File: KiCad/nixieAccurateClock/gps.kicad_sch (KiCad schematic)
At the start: 5 parts, among them J5 Conn_Coaxial, J6 Conn_01x02_Pin, U4 PX1125T

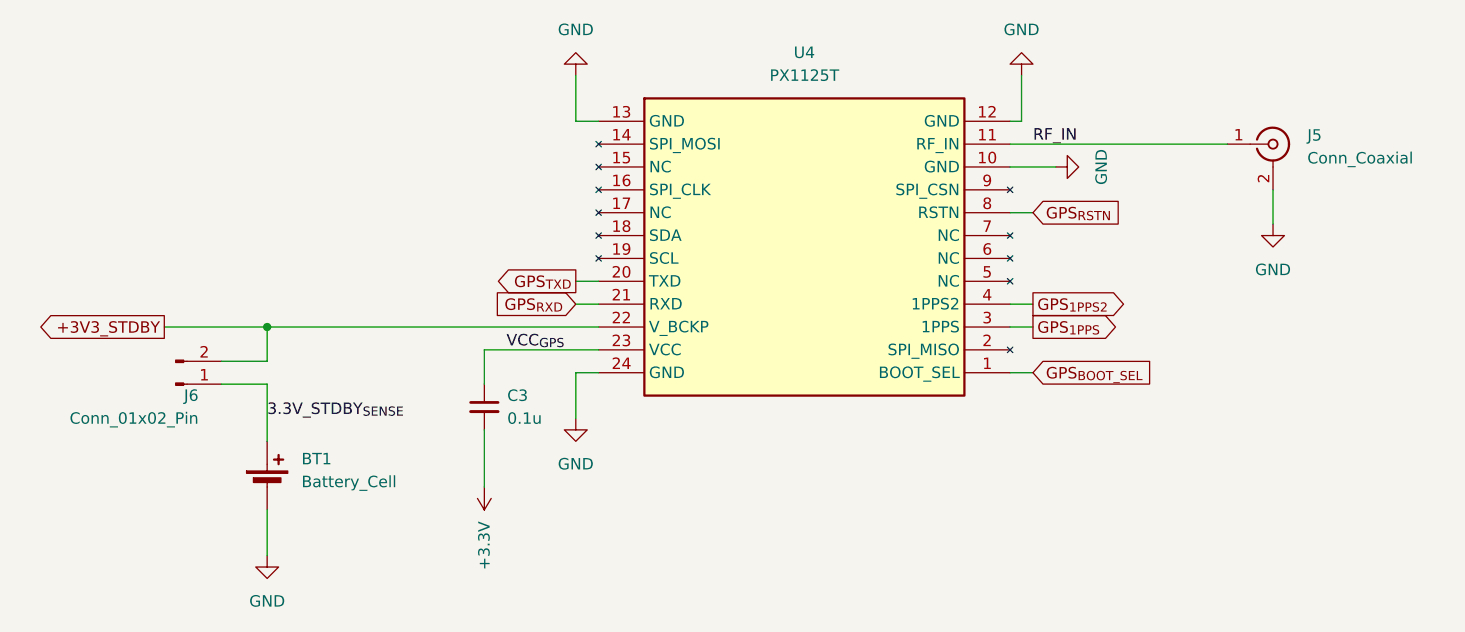
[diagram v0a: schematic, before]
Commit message: switch to 27k R_anode
Add voltage rail jumpers for different 5V and 3.3V standby applications
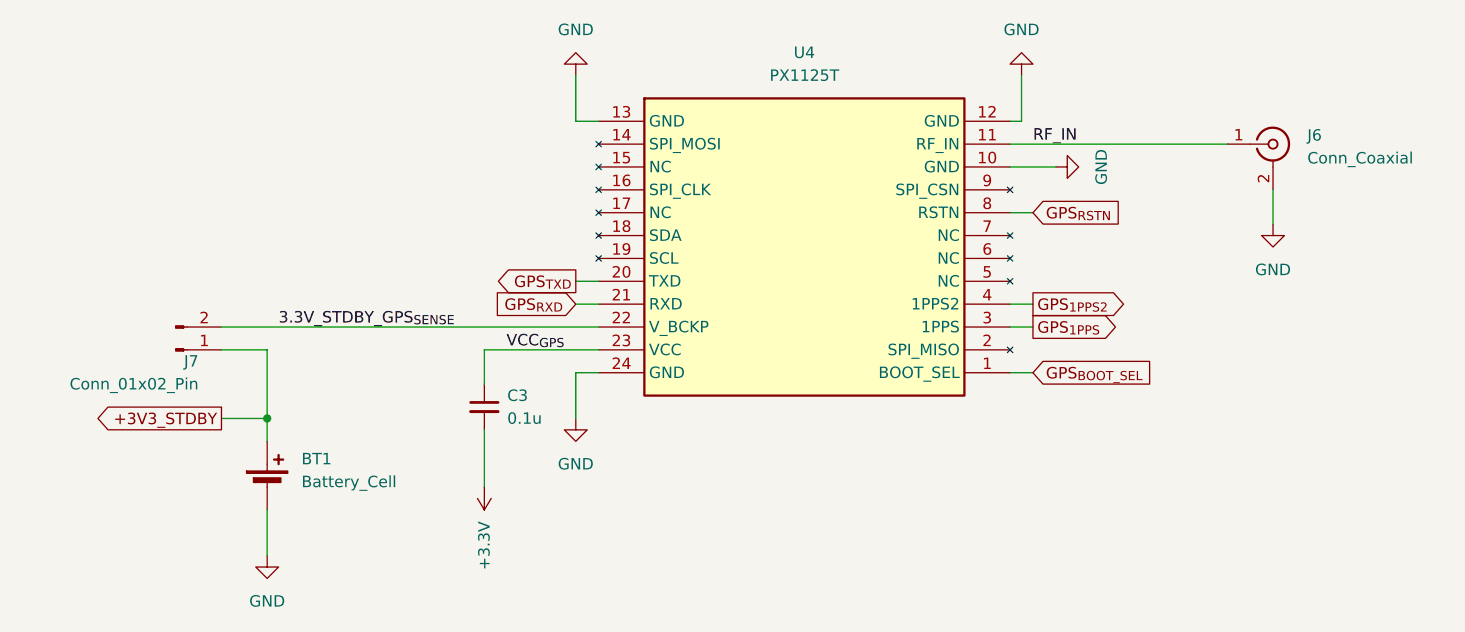
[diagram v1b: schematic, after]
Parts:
- renumbered J5 to J6, J6 to J7
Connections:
- net 3.3V_STDBY_{SENSE} is gone; now on net +3V3_STDBY: BT1.1 (+), J7.1 (Pin_1)
- net +3V3_STDBY: no longer J7.2 (Pin_2), U4.22 (V_BCKP)
- new net 3.3V_STDBY_GPS_{SENSE}: J7.2 (Pin_2), U4.22 (V_BCKP)
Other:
- moved on the sheet: J7
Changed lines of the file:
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@@
     (company "Paul Willis")
   )
-  (junction (at 72.39 110.49) (diameter 0) (color 0 0 0 0)
+  (junction (at 72.39 120.65) (diameter 0) (color 0 0 0 0)
   )
   (wire (pts (xy 184.15 95.25) (xy 184.15 99.06))
@@
     (stroke (width 0) (type default))
   )
-  (wire (pts (xy 72.39 110.49) (xy 109.22 110.49))
-    (stroke (width 0) (type default))
-  )
-  (wire (pts (xy 60.96 110.49) (xy 72.39 110.49))
-    (stroke (width 0) (type default))
-  )
   (wire (pts (xy 154.94 87.63) (xy 156.21 87.63))
     (stroke (width 0) (type default))
   )
-  (wire (pts (xy 72.39 114.3) (xy 72.39 110.49))
-    (stroke (width 0) (type default))
-  )
   (wire (pts (xy 72.39 130.81) (xy 72.39 135.89))
     (stroke (width 0) (type default))
@@
     (stroke (width 0) (type default))
   )
+  (wire (pts (xy 67.31 120.65) (xy 72.39 120.65))
+    (stroke (width 0) (type default))
+  )
+  (wire (pts (xy 67.31 110.49) (xy 109.22 110.49))
+    (stroke (width 0) (type default))
+  )
   (wire (pts (xy 154.94 110.49) (xy 157.48 110.49))
     (stroke (width 0) (type default))
@@
     (stroke (width 0) (type default))
   )
-  (wire (pts (xy 72.39 116.84) (xy 67.31 116.84))
-    (stroke (width 0) (type default))
-  )
-  (wire (pts (xy 67.31 114.3) (xy 72.39 114.3))
+  (wire (pts (xy 72.39 113.03) (xy 67.31 113.03))
+    (stroke (width 0) (type default))
+  )
+  (wire (pts (xy 72.39 120.65) (xy 72.39 123.19))
     (stroke (width 0) (type default))
   )
@@
     (stroke (width 0) (type default))
   )
-  (wire (pts (xy 72.39 116.84) (xy 72.39 123.19))
+  (wire (pts (xy 72.39 113.03) (xy 72.39 120.65))
     (stroke (width 0) (type default))
   )
@@
     (effects (font (size 1.27 1.27)) (justify right bottom))
   )
-  (label "3.3V_STDBY_{SENSE}" (at 72.39 120.65 0) (fields_autoplaced)
+  (label "3.3V_STDBY_GPS_{SENSE}" (at 73.66 110.49 0) (fields_autoplaced)
     (effects (font (size 1.27 1.27)) (justify left bottom))
   )
@@
     )
   )
-  (global_label "+3V3_STDBY" (shape output) (at 60.96 110.49 180) (fields_autoplaced)
+  (global_label "+3V3_STDBY" (shape output) (at 67.31 120.65 180) (fields_autoplaced)
     (effects (font (size 1.27 1.27)) (justify right))
-    (property "Intersheetrefs" "${INTERSHEET_REFS}" (at 46.1215 110.49 0)
+    (property "Intersheetrefs" "${INTERSHEET_REFS}" (at 52.4715 120.65 0)
       (effects (font (size 1.27 1.27)) (justify right) hide)
     )
@@
     )
   )
-  (symbol (lib_id "Connector:Conn_01x02_Pin") (at 62.23 116.84 0) (mirror x) (unit 1)
-    (in_bom yes) (on_board yes) (dnp no)
-    (property "Reference" "J6" (at 64.77 118.11 0)
+  (symbol (lib_id "Connector:Conn_01x02_Pin") (at 62.23 113.03 0) (mirror x) (unit 1)
+    (in_bom yes) (on_board yes) (dnp no)
+    (property "Reference" "J7" (at 64.77 114.3 0)
       (effects (font (size 1.27 1.27)) (justify right))
     )
-    (property "Value" "Conn_01x02_Pin" (at 64.77 120.65 0)
+    (property "Value" "Conn_01x02_Pin" (at 64.77 116.84 0)
       (effects (font (size 1.27 1.27)) (justify right))
     )
-    (property "Footprint" "Connector_PinHeader_2.54mm:PinHeader_1x02_P2.54mm_Vertical" (at 62.23 116.84 0)
-      (effects (font (size 1.27 1.27)) hide)
-    )
-    (property "Datasheet" "https://app.adam-tech.com/products/download/data_sheet/201605/ph1-xx-ua-data-sheet.pdf" (at 62.23 116.84 0)
-      (effects (font (size 1.27 1.27)) hide)
-    )
-    (property "Sim.Enable" "0" (at 62.23 116.84 0)
-      (effects (font (size 1.27 1.27)) hide)
-    )
-    (property "Model" "PH1-02-UA" (at 62.23 116.84 0)
-      (effects (font (size 1.27 1.27)) hide)
-    )
-    (property "Price" "0.10" (at 62.23 116.84 0)
-      (effects (font (size 1.27 1.27)) hide)
-    )
-    (property "Digikey link" "https://www.digikey.com/en/products/detail/adam-tech/PH1-02-UA/9830266" (at 62.23 116.84 0)
-      (effects (font (size 1.27 1.27)) hide)
-    )
-    (property "Mouser link" "https://www.mouser.com/ProductDetail/Samtec/TSW-102-07-G-S?qs=iT52DjcXudsNPhlNCDp8vw%3D%3D" (at 62.23 116.84 0)
+    (property "Footprint" "Connector_PinHeader_2.54mm:PinHeader_1x02_P2.54mm_Vertical" (at 62.23 113.03 0)
+      (effects (font (size 1.27 1.27)) hide)
+    )
+    (property "Datasheet" "https://app.adam-tech.com/products/download/data_sheet/201605/ph1-xx-ua-data-sheet.pdf" (at 62.23 113.03 0)
+      (effects (font (size 1.27 1.27)) hide)
+    )
+    (property "Sim.Enable" "0" (at 62.23 113.03 0)
+      (effects (font (size 1.27 1.27)) hide)
+    )
+    (property "Model" "PH1-02-UA" (at 62.23 113.03 0)
+      (effects (font (size 1.27 1.27)) hide)
+    )
+    (property "Price" "0.10" (at 62.23 113.03 0)
+      (effects (font (size 1.27 1.27)) hide)
+    )
+    (property "Digikey link" "https://www.digikey.com/en/products/detail/adam-tech/PH1-02-UA/9830266" (at 62.23 113.03 0)
+      (effects (font (size 1.27 1.27)) hide)
+    )
+    (property "Mouser link" "https://www.mouser.com/ProductDetail/Samtec/TSW-102-07-G-S?qs=iT52DjcXudsNPhlNCDp8vw%3D%3D" (at 62.23 113.03 0)
       (effects (font (size 1.27 1.27)) hide)
     )
@@
       (project "nixieAccurateClock"
         (path "/55aab698-7558-4fe2-95ad-faa6da60ef89/9610945c-9df3-4d66-a574-d19433fdc707"
-          (reference "J6") (unit 1)
+          (reference "J7") (unit 1)
         )
       )
@@
   (symbol (lib_id "Connector:Conn_Coaxial") (at 184.15 90.17 0) (unit 1)
     (in_bom yes) (on_board yes) (dnp no) (fields_autoplaced)
-    (property "Reference" "J5" (at 187.96 89.1932 0)
+    (property "Reference" "J6" (at 187.96 89.1932 0)
       (effects (font (size 1.27 1.27)) (justify left))
     )
@@
       (project "nixieAccurateClock"
         (path "/55aab698-7558-4fe2-95ad-faa6da60ef89/9610945c-9df3-4d66-a574-d19433fdc707"
-          (reference "J5") (unit 1)
-        )
-      )
+          (reference "J6") (unit 1)
+        )
+      )
